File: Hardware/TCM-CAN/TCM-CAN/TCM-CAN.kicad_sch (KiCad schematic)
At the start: 4 parts, among them J1 DTM13-12PA, J2 Conn_01x27_Socket, J3 Conn_01x27_Socket, J4 Conn_02x20_Odd_Even

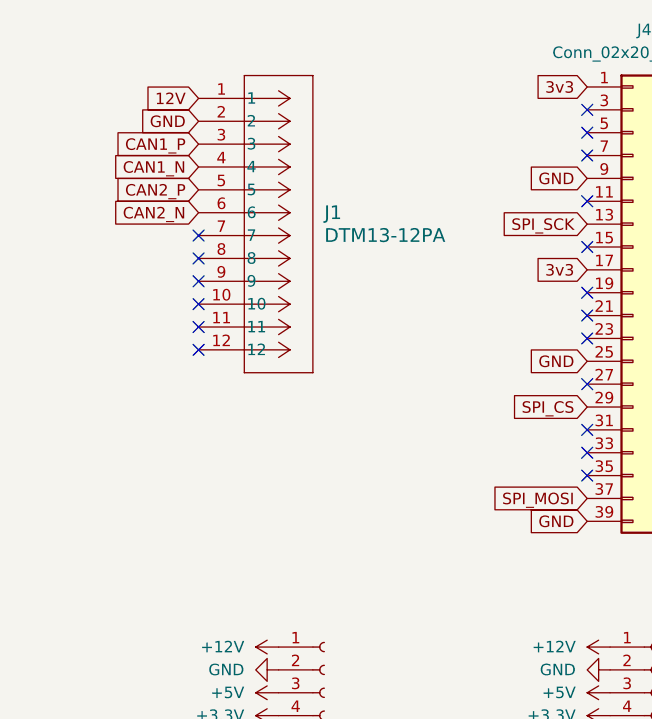
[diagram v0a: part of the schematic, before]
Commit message: bug fix
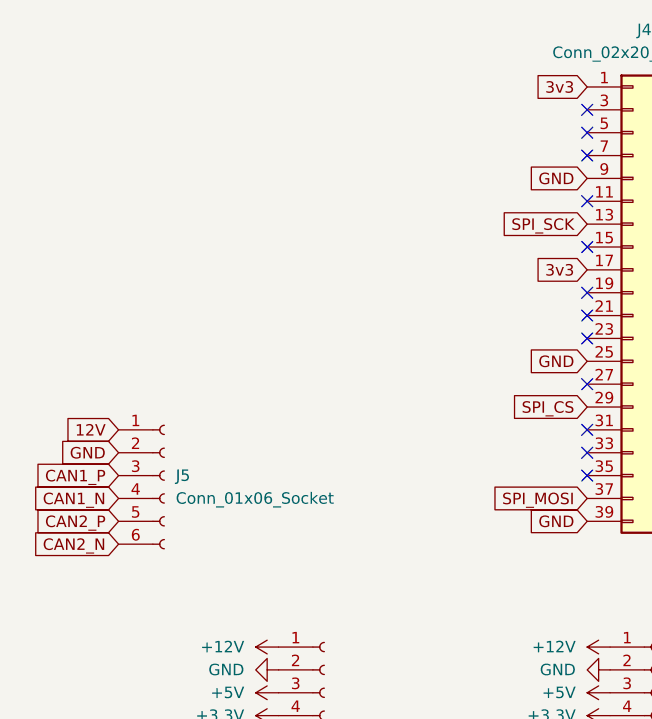
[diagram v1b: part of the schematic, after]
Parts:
- removed J1: DTM13-12PA, CONN12_DTM13-12PA_TEC, symbol DTM:DTM13-12PA
- added J5: Conn_01x06_Socket, Connector_JST:JST_XH_B6B-XH-A_1x06_P2.50mm_Vertical, symbol Connector:Conn_01x06_Socket
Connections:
- net 12V: now also J5.1 (Pin_1)
- net CAN1_N: now also J5.4 (Pin_4)
- net CAN1_P: now also J5.3 (Pin_3)
- net CAN2_N: now also J5.6 (Pin_6)
- net CAN2_P: now also J5.5 (Pin_5)
- net GND: now also J5.2 (Pin_2)
- no-connect marks 68 -> 62
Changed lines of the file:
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@@
 	)
 	(no_connect
-		(at 171.45 36.83)
-	)
-	(no_connect
 		(at 227.33 62.23)
 	)
@@
 	)
 	(no_connect
-		(at 171.45 49.53)
-	)
-	(no_connect
 		(at 180.34 125.73)
 	)
@@
 	)
 	(no_connect
-		(at 171.45 41.91)
-	)
-	(no_connect
 		(at 217.17 113.03)
 	)
@@
 	)
 	(no_connect
-		(at 171.45 44.45)
-	)
-	(no_connect
 		(at 214.63 27.94)
 	)
@@
 	)
 	(no_connect
-		(at 171.45 39.37)
-	)
-	(no_connect
 		(at 227.33 38.1)
 	)
 	(no_connect
-		(at 171.45 46.99)
-	)
-	(no_connect
 		(at 217.17 138.43)
 	)
@@
 			"AAAAAAAAAAAAAAAAAAAAAAAAAAAAAAAAAAAAAAAAAAAAAAAAAAAAAAAAAAAAAAAAAAAAAAAAAAAA"
 			"AAAAAAAAAAAAAAAAAAAAAAAAAAAAAAAAAAAAAAAAAAAAAAAAAAAAAAAAAAAAAAAAAAAAAAAAAAAA"
-			"AAAAAAAAAAAAAAAAAAAAAAAAAAAAAAAAAAAAAAA="
+			"AAAAAAAAAAAAAAAAAAAAAAAAAAAAAAAAAAAAAAAAAAAAAAAAAAAAAAAAAAAAAAAAAAAAAAAAAAAA"
+			"AAAAAAAAAAAAAAAAAAAAAAAAAAAAAAAAAAAAAAAAAAAAAAAAAAAAAAAAAAAAAAAAAAAAAAAAAAAA"
+			"AAAAAAAAAAAAAAAAAAAAAAAAAAAAAAAAAAAAAAAAAAAAAAAAAAAAAAAAAAAAAAAAAAAAAAAAAAAA"
+			"AAAAAAAAAAAAAAAAAAAAAAAAAAAAAAAAAAAAAAAAAAAAAAAAAAAAAAAAAAAAAAAAAAAAAAAAAAAA"
+			"AAAAAAAAAAAAAAAAAAAAAAAAAAAAAAAAAAAAAAAAAAAAAAAAAAAAAAAAAAAAAAAAAAAAAAAAAAAA"
+			"AAAAAAAAAAAAAAAAAAAAAAAAAAAAAAAAAAAAAAAAAAAAAAAAAAAAAAAAAAAAAAAAAAAAAAAAAAAA"
+			"AAAAAAAAAAAAAAAAAAAAAAAAAAAAAAAAAAAAAAAAAAAAAAAAAAAAAAAAAAAAAAAAAAAAAAAAAAAA"
+			"AAAAAAAAAAAAAAAAAAAAAAAAAAAAAAAAAAAAAAAAAAAAAAAAAAAAAAAAAAAAAAAAAAAAAAAAAAAA"
+			"AAAAAAAAAAAAAAAAAAAAAAAAAAAAAAAAAAAAAAAAAAAAAAAAAAAAAAAAAAAAAAAAAAAAAAAAAAAA"
+			"AAAAAAAAAAAAAAAAAAAAAAAAAAAAAAAAAAAAAAAAAAAAAAAAAAAAAAAAAAAAAAAAAAAAAAAAAAAA"
+			"AAAAAAAAAAAAAAAAAAAAAAAAAAAAAAAAAAAAAAAAAAAAAAAAAAAAAAAAAAAAAAAAAAAAAAAAAAAA"
+			"AAAAAAAAAAAAAAAAAAAAAAAAAAAAAAAAAAAAAAAAAAAAAAAAAAAAAAAAAAAAAAAAAAAAAAAAAAAA"
+			"AAAAAAAAAAAAAAAAAAAAAAAAAAAAAAAAAAAAAAAAAAAAAAAAAAAAAAAAAAAAAAAAAAAAAAAAAAAA"
+			"AAAAAAAAAAAAAAAAAAAAAAAAAAAAAAAAAAAAAAAAAAAAAAAAAAAAAAAAAAAAAAAAAAAAAAAAAAAA"
+			"AAAAAAAAAAAAAAAAAAAAAAAAAAAAAAAAAAAAAAAAAAAAAAAAAAAAAAAAAAAAAAAAAAAAAAAAAAAA"
+			"AAAAAAAAAAAAAAAAAAAAAAAAAAAAAAAAAAAAAAAAAAAAAAAAAAAAAAAAAAAAAAAAAAAAAAAAAAAA"
+			"AAAAAAAAAAAAAAAAAAAAAAAAAAAAAAAAAAAAAAAAAAAAAAAAAAAAAAAAAAAAAAAAAAAAAAAAAAAA"
+			"AAAAAAAAAAAAAAAAAAAAAAAAAAAAAAAAAAAAAAAAAAAAAAAAAAAAAAAAAAAAAAAAAAAAAAAAAAAA"
+			"AAAAAAAAAAAAAAAAAAAAAAAAAAAAAAAAAAAAAA=="
 		)
 	)
@@
 		)
 	)
-	(global_label "3v3"
+	(global_label "CAN2_N"
 		(shape input)
-		(at 214.63 40.64 180)
+		(at 162.56 71.12 180)
 		(fields_autoplaced yes)
 		(effects
@@
 		)
 		(property "Intersheetrefs" "${INTERSHEET_REFS}"
-			(at 208.2582 40.64 0)
+			(at 152.3781 71.12 0)
 			(effects
 				(font
@@
 		)
 	)
-	(global_label "12V"
+	(global_label "CAN1_P"
+		(shape input)
+		(at 162.56 63.5 180)
+		(fields_autoplaced yes)
+		(effects
+			(font
+				(size 1.27 1.27)
+			)
+			(justify right)
+		)
+		(property "Intersheetrefs" "${INTERSHEET_REFS}"
+			(at 152.4386 63.5 0)
+			(effects
+				(font
+					(size 1.27 1.27)
+				)
+				(justify right)
+				(hide yes)
+			)
+		)
+	)
+	(global_label "3v3"
 		(shape input)
-		(at 171.45 21.59 180)
+		(at 214.63 40.64 180)
 		(fields_autoplaced yes)
 		(effects
@@
 		)
 		(property "Intersheetrefs" "${INTERSHEET_REFS}"
-			(at 164.9572 21.59 0)
+			(at 208.2582 40.64 0)
 			(effects
 				(font
@@
 	(global_label "GND"
 		(shape input)
-		(at 171.45 24.13 180)
+		(at 162.56 60.96 180)
 		(fields_autoplaced yes)
 		(effects
@@
 		)
 		(property "Intersheetrefs" "${INTERSHEET_REFS}"
-			(at 164.5943 24.13 0)
+			(at 155.7043 60.96 0)
 			(effects
 				(font
@@
 		)
 	)
-	(global_label "CAN2_P"
-		(shape input)
-		(at 171.45 31.75 180)
-		(fields_autoplaced yes)
-		(effects
-			(font
-				(size 1.27 1.27)
-			)
-			(justify right)
-		)
-		(property "Intersheetrefs" "${INTERSHEET_REFS}"
-			(at 161.3286 31.75 0)
-			(effects
-				(font
-					(size 1.27 1.27)
-				)
-				(justify right)
-				(hide yes)
-			)
-		)
-	)
 	(global_label "SPI_MOSI"
 		(shape input)
@@
 		)
 	)
-	(global_label "CAN1_P"
-		(shape input)
-		(at 171.45 26.67 180)
-		(fields_autoplaced yes)
-		(effects
-			(font
-				(size 1.27 1.27)
-			)
-			(justify right)
-		)
-		(property "Intersheetrefs" "${INTERSHEET_REFS}"
-			(at 161.3286 26.67 0)
-			(effects
-				(font
-					(size 1.27 1.27)
-				)
-				(justify right)
-				(hide yes)
-			)
-		)
-	)
-	(global_label "CAN2_N"
+	(global_label "CAN1_N"
 		(shape input)
-		(at 171.45 34.29 180)
+		(at 162.56 66.04 180)
 		(fields_autoplaced yes)
 		(effects
@@
 		)
 		(property "Intersheetrefs" "${INTERSHEET_REFS}"
-			(at 161.2681 34.29 0)
+			(at 152.3781 66.04 0)
 			(effects
 				(font
@@
 		)
 	)
-	(global_label "CAN1_N"
+	(global_label "PA4"
 		(shape input)
-		(at 171.45 29.21 180)
+		(at 180.34 138.43 180)
 		(fields_autoplaced yes)
 		(effects
@@
 		)
 		(property "Intersheetrefs" "${INTERSHEET_REFS}"
-			(at 161.2681 29.21 0)
+			(at 173.7867 138.43 0)
 			(effects
 				(font
@@
 		)
 	)
-	(global_label "PA4"
+	(global_label "SPI1_SCK"
 		(shape input)
-		(at 180.34 138.43 180)
+		(at 180.34 135.89 180)
 		(fields_autoplaced yes)
 		(effects
@@
 		)
 		(property "Intersheetrefs" "${INTERSHEET_REFS}"
-			(at 173.7867 138.43 0)
+			(at 168.3439 135.89 0)
 			(effects
 				(font
@@
 		)
 	)
-	(global_label "SPI1_SCK"
+	(global_label "CAN2_P"
 		(shape input)
-		(at 180.34 135.89 180)
+		(at 162.56 68.58 180)
 		(fields_autoplaced yes)
 		(effects
@@
 		)
 		(property "Intersheetrefs" "${INTERSHEET_REFS}"
-			(at 168.3439 135.89 0)
+			(at 152.4386 68.58 0)
 			(effects
 				(font
@@
 		)
 	)
-	(global_label "GND"
+	(global_label "12V"
 		(shape input)
-		(at 214.63 30.48 180)
+		(at 162.56 58.42 180)
 		(fields_autoplaced yes)
 		(effects
@@
 		)
 		(property "Intersheetrefs" "${INTERSHEET_REFS}"
-			(at 207.7743 30.48 0)
+			(at 156.0672 58.42 0)
 			(effects
 				(font
@@
 	(global_label "GND"
 		(shape input)
-		(at 227.33 43.18 0)
+		(at 214.63 30.48 180)
 		(fields_autoplaced yes)
 		(effects
@@
 				(size 1.27 1.27)
 			)
-			(justify left)
+			(justify right)
 		)
 		(property "Intersheetrefs" "${INTERSHEET_REFS}"
-			(at 234.1857 43.18 0)
+			(at 207.7743 30.48 0)
 			(effects
 				(font
 					(size 1.27 1.27)
 				)
-				(justify left)
+				(justify right)
 				(hide yes)
 			)
 		)
 	)
-	(symbol
-		(lib_id "DTM:DTM13-12PA")
-		(at 181.61 36.83 0)
-		(unit 1)
-		(exclude_from_sim no)
-		(in_bom yes)
-		(on_board yes)
-		(dnp no)
+	(global_label "GND"
+		(shape input)
+		(at 227.33 43.18 0)
 		(fields_autoplaced yes)
-		(property "Reference" "J1"
-			(at 185.42 34.2899 0)
-			(effects
-				(font
-					(size 1.524 1.524)
-				)
-				(justify left)
-			)
-		)
-		(property "Value" "DTM13-12PA"
-			(at 185.42 36.8299 0)
-			(effects
-				(font
-					(size 1.524 1.524)
-				)
-				(justify left)
-			)
-		)
-		(property "Footprint" "CONN12_DTM13-12PA_TEC"
-			(at 181.61 36.83 0)
-			(effects
-				(font
-					(size 1.27 1.27)
-					(italic yes)
-				)
-				(hide yes)
-			)
-		)
-		(property "Datasheet" "DTM13-12PA"
-			(at 181.61 36.83 0)
-			(effects
-				(font
-					(size 1.27 1.27)
-					(italic yes)
-				)
-				(hide yes)
+		(effects
+			(font
+				(size 1.27 1.27)
 			)
+			(justify left)
 		)
-		(property "Description" ""
-			(at 181.61 36.83 0)
+		(property "Intersheetrefs" "${INTERSHEET_REFS}"
+			(at 234.1857 43.18 0)
 			(effects
 				(font
 					(size 1.27 1.27)
 				)
+				(justify left)
 				(hide yes)
 			)
 		)
-		(pin "8"
-		)
-		(pin "3"
-		)
-		(pin "6"
-		)
-		(pin "4"
-		)
-		(pin "1"
-		)
-		(pin "12"
-		)
-		(pin "10"
-		)
-		(pin "5"
-		)
-		(pin "9"
-		)
-		(pin "2"
-		)
-		(pin "7"
-		)
-		(pin "11"
-		)
-		(instances
-			(project ""
-				(path "/dce5d582-08ac-45e6-8e98-75b83df6efb2"
-					(reference "J1")
-					(unit 1)
-				)
-			)
-		)
 	)
 	(symbol
@@
 					(unit 1)
 				)
+			)
+		)
+	)
+	(symbol
+		(lib_id "Connector:Conn_01x06_Socket")
+		(at 167.64 63.5 0)
+		(unit 1)
+		(exclude_from_sim no)
+		(in_bom yes)
+		(on_board yes)
+		(dnp no)
+		(fields_autoplaced yes)
+		(property "Reference" "J5"
+			(at 168.91 63.4999 0)
+			(effects
+				(font
+					(size 1.27 1.27)
+				)
+				(justify left)
+			)
+		)
+		(property "Value" "Conn_01x06_Socket"
+			(at 168.91 66.0399 0)
+			(effects
+				(font
+					(size 1.27 1.27)
+				)
+				(justify left)
+			)
+		)
+		(property "Footprint" "Connector_JST:JST_XH_B6B-XH-A_1x06_P2.50mm_Vertical"
+			(at 167.64 63.5 0)
+			(effects
+				(font
+					(size 1.27 1.27)
+				)
+				(hide yes)
+			)
+		)
+		(property "Datasheet" "~"
+			(at 167.64 63.5 0)
+			(effects
+				(font
+					(size 1.27 1.27)
+				)
+				(hide yes)
+			)
+		)
+		(property "Description" "Generic connector, single row, 01x06, script generated"
+			(at 167.64 63.5 0)
+			(effects
+				(font
+					(size 1.27 1.27)
+				)
+				(hide yes)
+			)
+		)
+		(pin "1"
+		)
+		(pin "6"
+		)
+		(pin "5"
+		)
+		(pin "4"
+		)
+		(pin "2"
+		)
+		(pin "3"
+		)
+		(instances
+			(project ""
+				(path "/dce5d582-08ac-45e6-8e98-75b83df6efb2"
+					(reference "J5")
+					(unit 1)
+				)
